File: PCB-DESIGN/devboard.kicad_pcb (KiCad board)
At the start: 2 copper layers, 21 x 51 mm, 34 parts, among them J1 USB_C_Receptacle_USB2.0_14P, J2 Conn_01x20, J3 Conn_01x20, J4 Conn_01x03, SW1 SW_Push, U1 RP2040, U2 MCP1700x-330xxTT, U3 W25Q16JVUXIQ TR, Y1 12 MHz

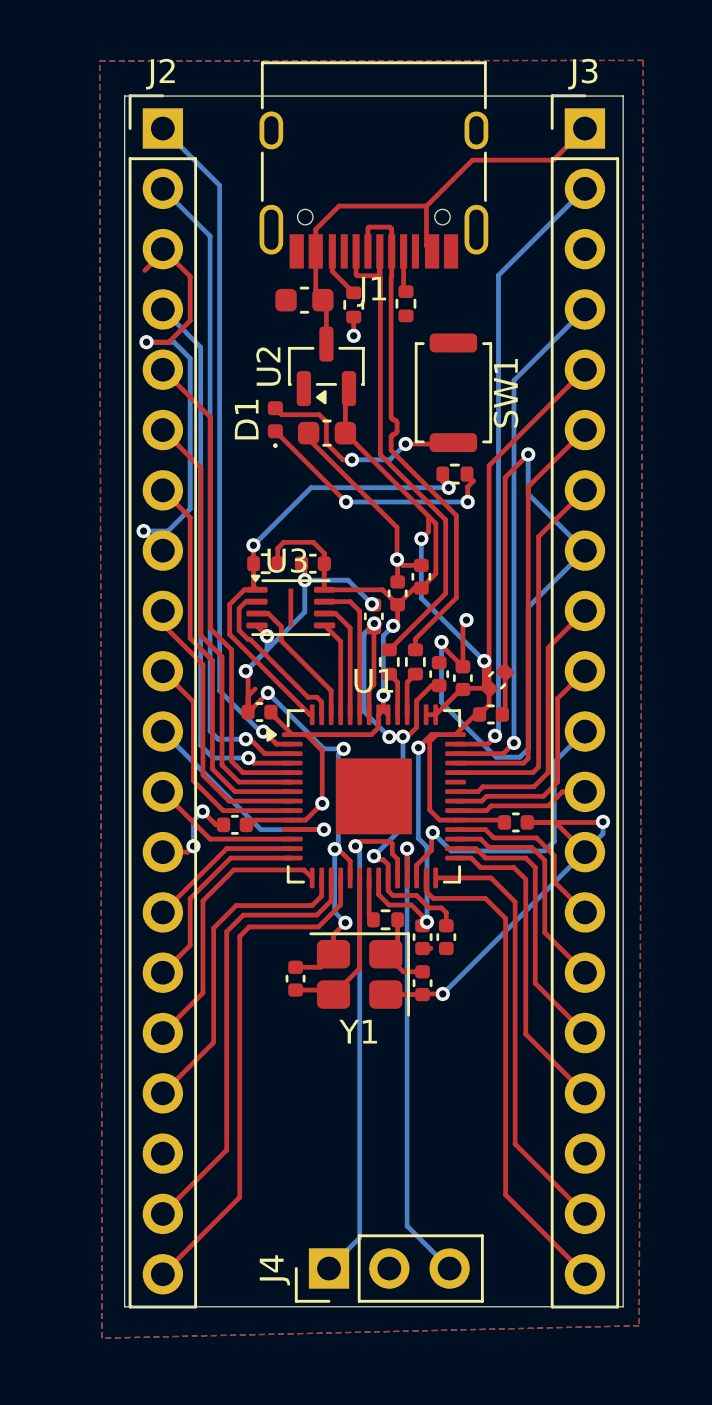
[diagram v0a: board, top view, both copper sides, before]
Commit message: Add files via upload
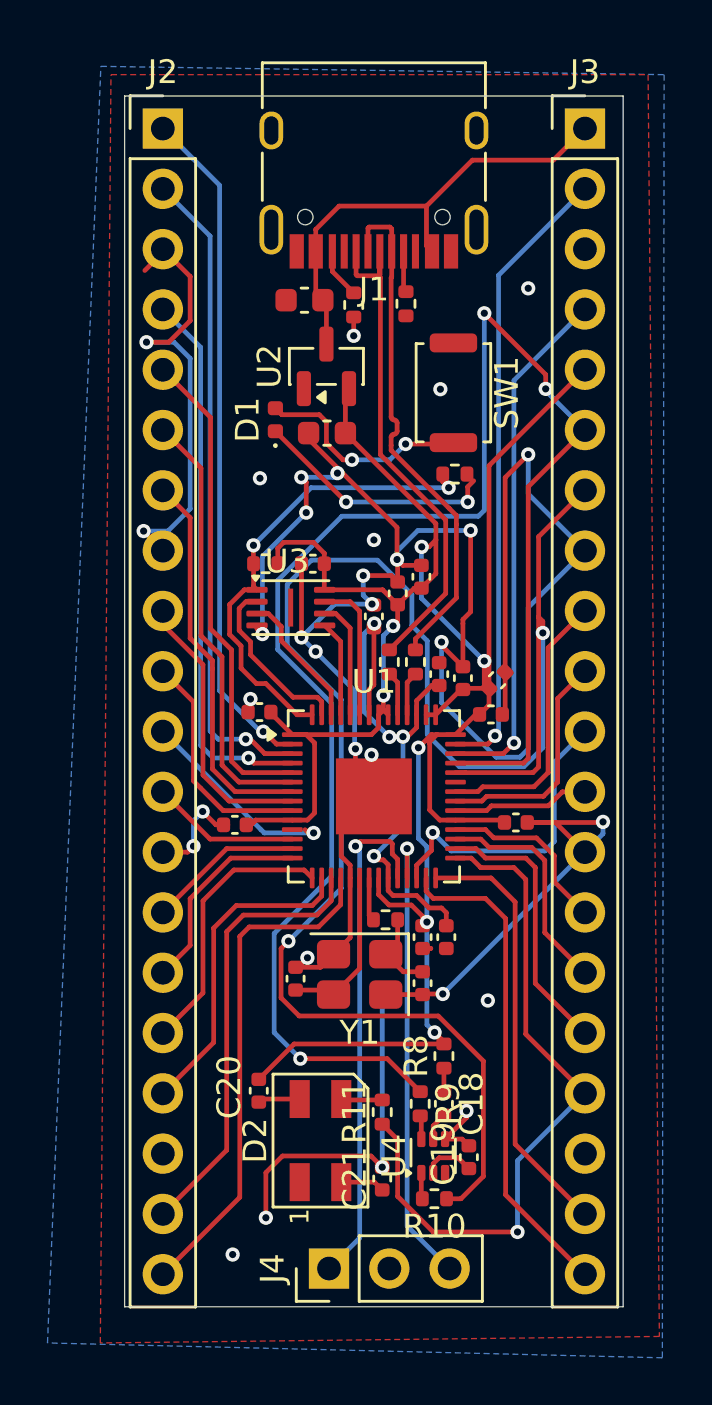
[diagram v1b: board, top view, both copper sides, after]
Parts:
- added C18: 0.1uF, Capacitor_SMD:C_0402_1005Metric, F.Cu at (162.9, 89.2)
- added C19: 0.1uF, Capacitor_SMD:C_0402_1005Metric, F.Cu at (164.0, 91.5)
- added C20: 0.1uF, Capacitor_SMD:C_0402_1005Metric, F.Cu at (155.2, 88.7)
- added C21: 0.1uF, Capacitor_SMD:C_0402_1005Metric, F.Cu at (160.3, 92.3)
- added D2: SK6812MINI, LED_SMD:LED_SK6812MINI_PLCC4_3.5x3.5mm_P1.75mm, F.Cu at (157.8, 90.8)
- added R10: 4.7k, Resistor_SMD:R_0402_1005Metric, F.Cu at (162.6, 93.2)
- added R11: 220, Resistor_SMD:R_0402_1005Metric, F.Cu at (160.3, 89.5)
- added R8: 4.7k, Resistor_SMD:R_0402_1005Metric, F.Cu at (162.9, 87.2)
- added R9: 4.7k, Resistor_SMD:R_0402_1005Metric, F.Cu at (161.9, 89.2)
- added U4: TMP112xxDRL, Package_TO_SOT_SMD:SOT-563, F.Cu at (162.5, 91.4)
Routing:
- net GPIO26_ADC0: track 16.1 -> 75.7 mm, vias 0 -> 2
- net GPIO27_ADC1: track 18.0 -> 71.0 mm, vias 0 -> 3
- net GND: track 121.0 -> 149.9 mm, vias 19 -> 32
- net GPIO18: track 13.4 -> 29.4 mm, vias 0 -> 1
- net +3V3: track 86.6 -> 99.6 mm
- net Net-(U4-GND): track 0.00 -> 2.18 mm
- net Net-(D2-VSS): track 0.00 -> 1.86 mm
- net Net-(D2-VDD): track 0.00 -> 1.78 mm
- net Net-(D2-DIN): track 0.00 -> 1.74 mm
- net GPIO8: track 10.0 -> 8.54 mm
- net Net-(U4-V+): track 0.00 -> 1.19 mm
- net Net-(U4-SCL): track 0.00 -> 1.11 mm
- net Net-(C18-Pad1): track 0.00 -> 1.02 mm
- net Net-(U4-SDA): track 0.00 -> 1.00 mm
- net QSPI_SS: track 19.4 -> 19.9 mm
